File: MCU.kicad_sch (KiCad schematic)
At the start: 34 parts, among them J1 F31L-1A7H1-11030, J17 Conn_02x30_Counter_Clockwise, J2 F31L-1A7H1-11030, J3 F31L-1A7H1-11030, J4 Conn_02x30_Counter_Clockwise, J6 Conn_01x02, U3 TPS76333, U4 TPS76333

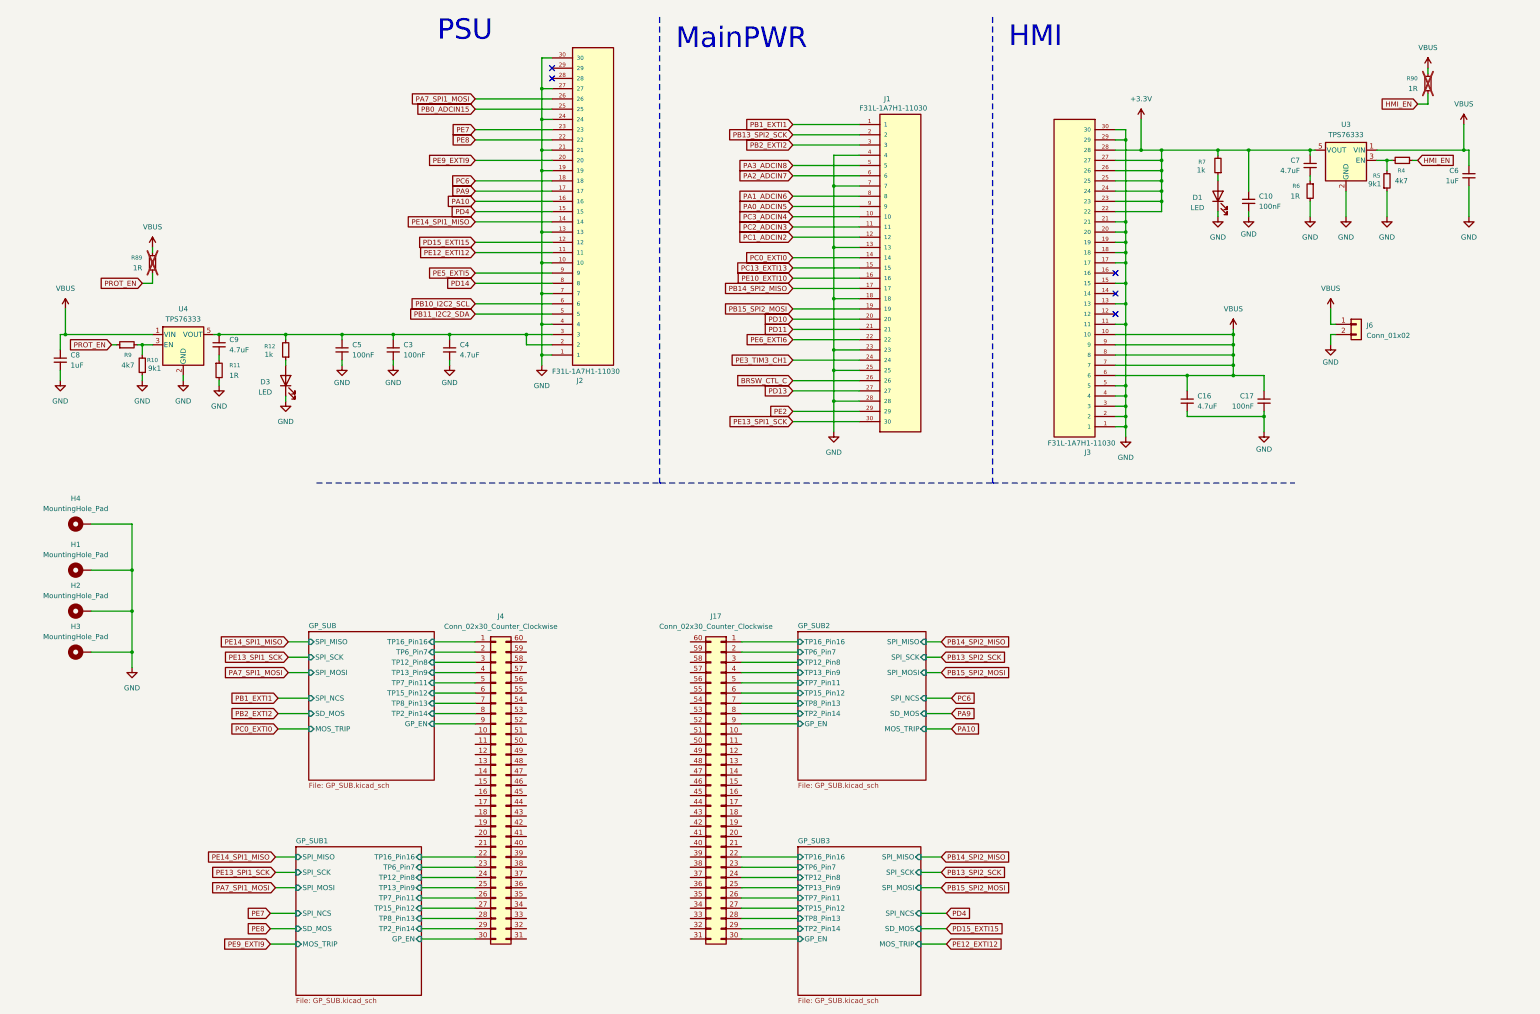
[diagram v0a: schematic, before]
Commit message: Add files via upload
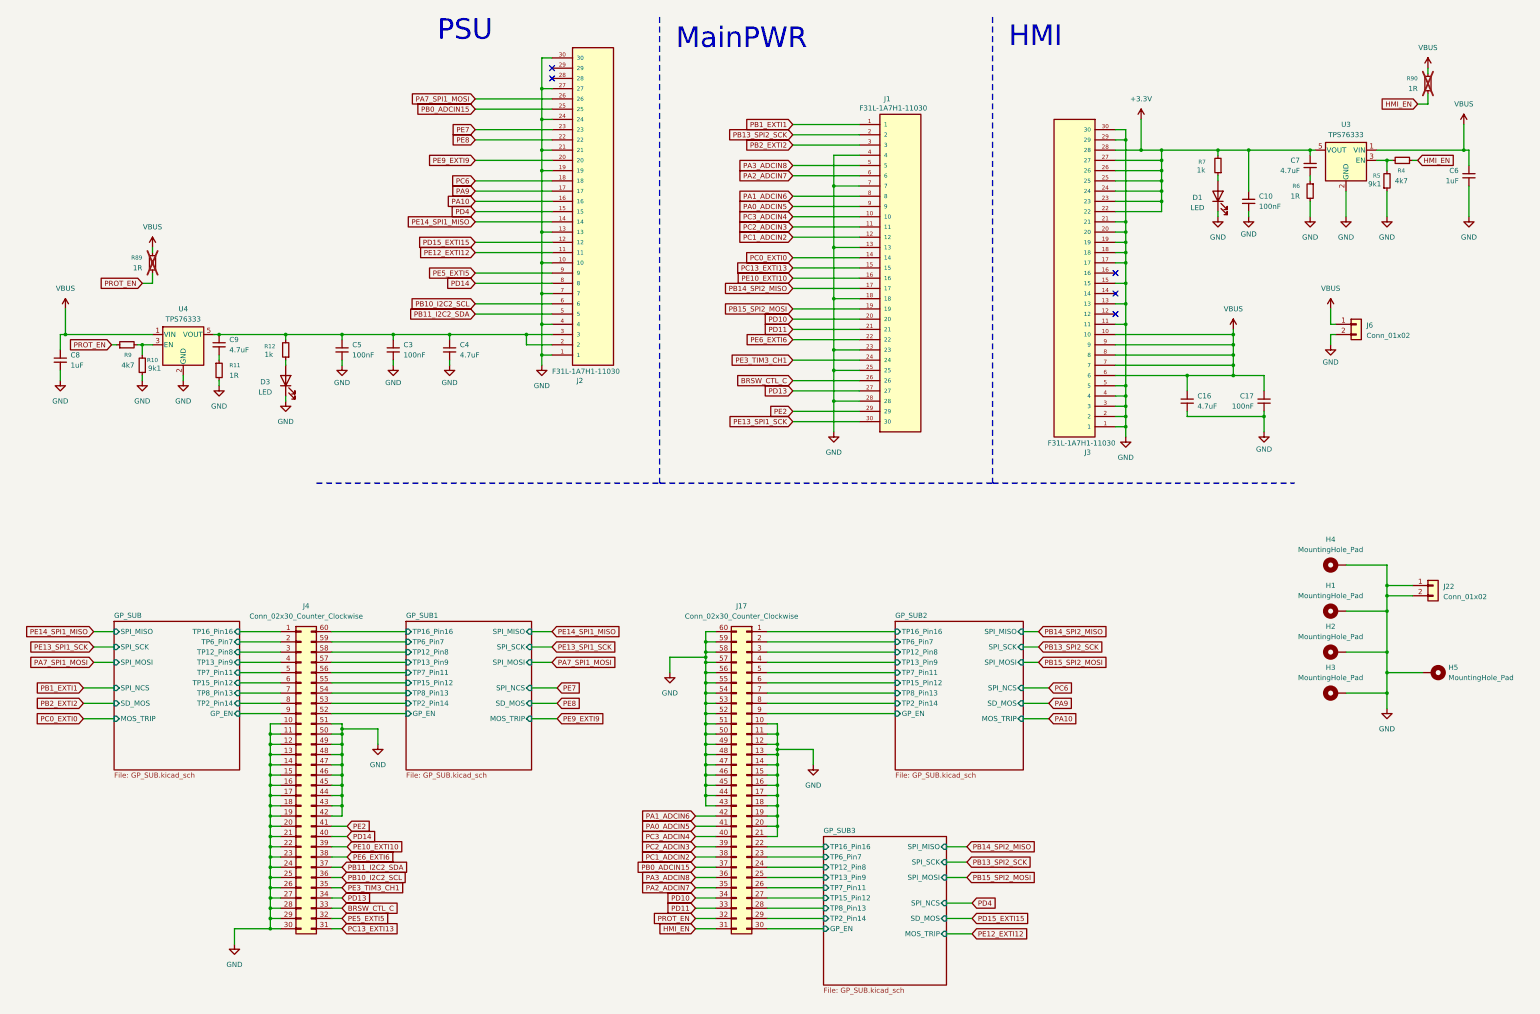
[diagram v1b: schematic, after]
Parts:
- added H5: MountingHole_Pad, MountingHole:MountingHole_2.2mm_M2_DIN965_Pad, symbol Mechanical:MountingHole_Pad
- added J22: Conn_01x02, Connector_PinHeader_2.54mm:PinHeader_1x02_P2.54mm_Vertical, symbol Connector_Generic:Conn_01x02
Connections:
- net BRSW_CTL_C: now also J4.33 (Pin_33)
- net GND: now also J17.10 (Pin_10), J17.11 (Pin_11), J17.12 (Pin_12), J17.13 (Pin_13), J17.14 (Pin_14), J17.15 (Pin_15), J17.16 (Pin_16), J17.17 (Pin_17), J17.18 (Pin_18), J17.19 (Pin_19), J17.20 (Pin_20), J17.21 (Pin_21), J17.43 (Pin_43), J17.44 (Pin_44), J17.45 (Pin_45), J17.46 (Pin_46), J17.47 (Pin_47), J17.48 (Pin_48), J17.49 (Pin_49), J17.50 (Pin_50), J17.51 (Pin_51), J17.52 (Pin_52), J17.53 (Pin_53), J17.54 (Pin_54), J17.55 (Pin_55), J17.56 (Pin_56), J17.57 (Pin_57), J17.58 (Pin_58), J17.59 (Pin_59), J17.60 (Pin_60), J4.10 (Pin_10), J4.11 (Pin_11), J4.12 (Pin_12), J4.13 (Pin_13), J4.14 (Pin_14), J4.15 (Pin_15), J4.16 (Pin_16), J4.17 (Pin_17), J4.18 (Pin_18), J4.19 (Pin_19), J4.20 (Pin_20), J4.21 (Pin_21), J4.22 (Pin_22), J4.23 (Pin_23), J4.24 (Pin_24), J4.25 (Pin_25), J4.26 (Pin_26), J4.27 (Pin_27), J4.28 (Pin_28), J4.29 (Pin_29), J4.30 (Pin_30), J4.42 (Pin_42), J4.43 (Pin_43), J4.44 (Pin_44), J4.45 (Pin_45), J4.46 (Pin_46), J4.47 (Pin_47), J4.48 (Pin_48), J4.49 (Pin_49), J4.50 (Pin_50), J4.51 (Pin_51), H5.1, J22.1 (Pin_1), J22.2 (Pin_2)
- net GP_SUB1/GP_EN: now also J4.52 (Pin_52); no longer J4.30 (Pin_30)
- net GP_SUB1/TP12_Pin8: now also J4.58 (Pin_58); no longer J4.24 (Pin_24)
- net GP_SUB1/TP13_Pin9: now also J4.57 (Pin_57); no longer J4.25 (Pin_25)
- net GP_SUB1/TP15_Pin12: now also J4.55 (Pin_55); no longer J4.27 (Pin_27)
- net GP_SUB1/TP16_Pin16: now also J4.60 (Pin_60); no longer J4.22 (Pin_22)
- net GP_SUB1/TP2_Pin14: now also J4.53 (Pin_53); no longer J4.29 (Pin_29)
- net GP_SUB1/TP6_Pin7: now also J4.59 (Pin_59); no longer J4.23 (Pin_23)
- net GP_SUB1/TP7_Pin11: now also J4.56 (Pin_56); no longer J4.26 (Pin_26)
- net GP_SUB1/TP8_Pin13: now also J4.54 (Pin_54); no longer J4.28 (Pin_28)
- net HMI_EN: now also J17.31 (Pin_31)
- net PA0_ADCIN5: now also J17.41 (Pin_41)
- net PA1_ADCIN6: now also J17.42 (Pin_42)
- net PA2_ADCIN7: now also J17.35 (Pin_35)
- net PA3_ADCIN8: now also J17.36 (Pin_36)
- net PB0_ADCIN15: now also J17.37 (Pin_37)
- net PB10_I2C2_SCL: now also J4.36 (Pin_36)
- net PB11_I2C2_SDA: now also J4.37 (Pin_37)
- net PC13_EXTI13: now also J4.31 (Pin_31)
- net PC1_ADCIN2: now also J17.38 (Pin_38)
- net PC2_ADCIN3: now also J17.39 (Pin_39)
- net PC3_ADCIN4: now also J17.40 (Pin_40)
- net PD10: now also J17.34 (Pin_34)
- net PD11: now also J17.33 (Pin_33)
- net PD13: now also J4.34 (Pin_34)
- net PD14: now also J4.40 (Pin_40)
- net PE10_EXTI10: now also J4.39 (Pin_39)
- net PE2: now also J4.41 (Pin_41)
- net PE3_TIM3_CH1: now also J4.35 (Pin_35)
- net PE5_EXTI5: now also J4.32 (Pin_32)
- net PE6_EXTI6: now also J4.38 (Pin_38)
- net PROT_EN: now also J17.32 (Pin_32)
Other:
- moved on the sheet: H1, H2, H3, H4, J17, J4
